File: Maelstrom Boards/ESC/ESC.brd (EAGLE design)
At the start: 101.6 x 101.6 mm, 54 parts, among them P5 MALE1PINHEADER, P6 MALE1PINHEADER, P7 MALE1PINHEADER, P8 MALE1PINHEADER

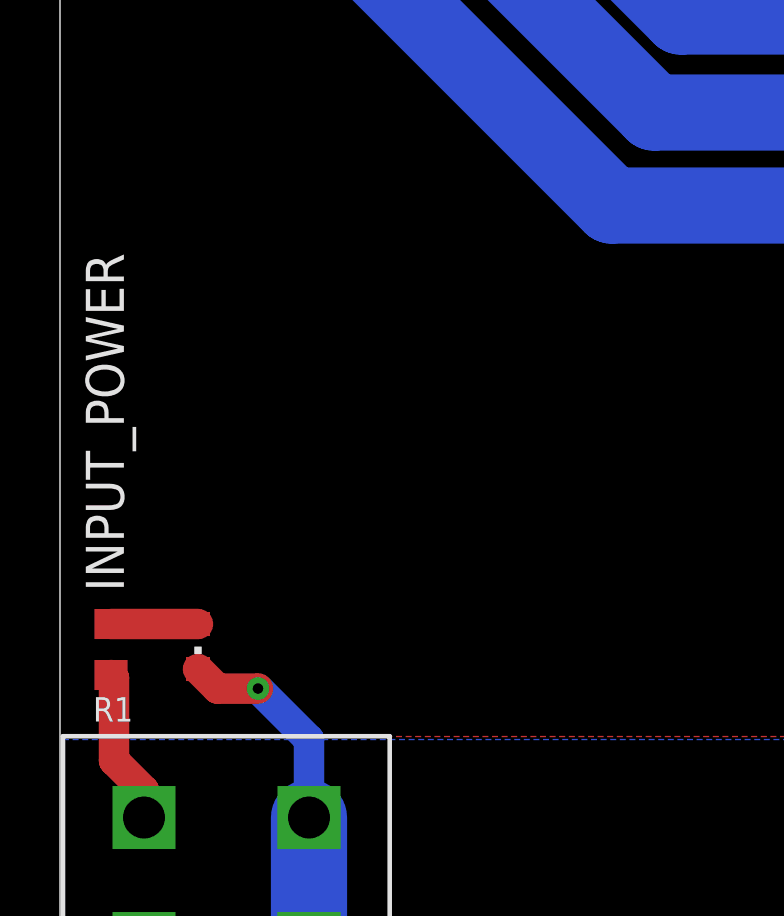
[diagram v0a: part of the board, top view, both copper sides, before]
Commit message: Final changes before order
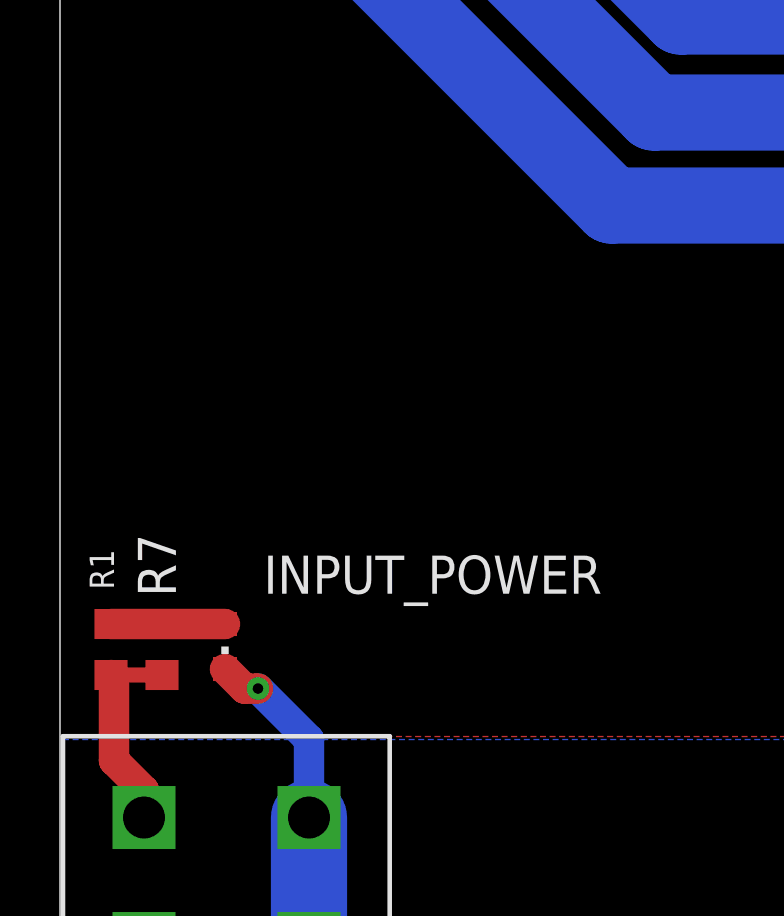
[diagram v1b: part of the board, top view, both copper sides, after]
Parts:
- added R7: 900, resistor:R0603
- R1: value (none) -> 900
- R2: value (none) -> 5
- R3, R4, R5, R6: value (none) -> 100k
- moved INPUT_POWER 0.90 mm to (5.50, 47.0)
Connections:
- net BALANCED+: now also R7.1
- net N$25: now also R7.2
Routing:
- net N$25: track 2.90 -> 5.50 mm
- net BALANCED+: track 5.21 -> 6.91 mm
- net GND: track 149.0 -> 148.1 mm
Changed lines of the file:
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@@
 <layer number="25" name="tNames" color="7" fill="1" visible="yes" active="yes"/>
 <layer number="26" name="bNames" color="7" fill="1" visible="yes" active="yes"/>
-<layer number="27" name="tValues" color="7" fill="1" visible="yes" active="yes"/>
-<layer number="28" name="bValues" color="7" fill="1" visible="yes" active="yes"/>
+<layer number="27" name="tValues" color="7" fill="1" visible="no" active="yes"/>
+<layer number="28" name="bValues" color="7" fill="1" visible="no" active="yes"/>
 <layer number="29" name="tStop" color="7" fill="3" visible="yes" active="yes"/>
 <layer number="30" name="bStop" color="7" fill="6" visible="yes" active="yes"/>
@@
 <text x="98.8" y="24.8" size="0.8128" layer="25">R4</text>
 <text x="30.7" y="8.8" size="0.8128" layer="25">R2</text>
-<text x="1.1" y="44.5" size="0.8128" layer="25">R1</text>
+<text x="1.8" y="48.9" size="0.8128" layer="25" rot="R90">R1</text>
 <text x="83.2" y="11.3" size="1.27" layer="26" rot="MR0">8</text>
 </plain>
@@
 <element name="P8" library="Male_Header_1Pin" package="MALE1PINHEADER" value="MALE1PINHEADER" x="82.55" y="9.652" smashed="yes" rot="R90"/>
 <element name="U$19" library="14_Pin_Connector_Vert" package="14PIN_VERT" value="14PIN_VERT" x="2.8" y="16.1" smashed="yes"/>
-<element name="R1" library="resistor" library_urn="urn:adsk.eagle:library:348" package="R0603" package3d_urn="urn:adsk.eagle:package:26057/1" value="" x="1.7" y="46.9" smashed="yes" rot="R90">
+<element name="R1" library="resistor" library_urn="urn:adsk.eagle:library:348" package="R0603" package3d_urn="urn:adsk.eagle:package:26057/1" value="900" x="1.7" y="46.9" smashed="yes" rot="R90">
 <attribute name="VALUE" x="3.605" y="46.265" size="1.27" layer="27" rot="R90"/>
 </element>
-<element name="R2" library="resistor" library_urn="urn:adsk.eagle:library:348" package="R0603" package3d_urn="urn:adsk.eagle:package:26057/1" value="" x="29.8" y="10.7" smashed="yes">
+<element name="R2" library="resistor" library_urn="urn:adsk.eagle:library:348" package="R0603" package3d_urn="urn:adsk.eagle:package:26057/1" value="5" x="29.8" y="10.7" smashed="yes">
 <attribute name="VALUE" x="29.165" y="8.795" size="1.27" layer="27"/>
 </element>
@@
 <attribute name="VALUE" x="31.53" y="8.795" size="1.27" layer="27"/>
 </element>
-<element name="INPUT_POWER" library="led" library_urn="urn:adsk.eagle:library:259" package="CHIPLED_0603" package3d_urn="urn:adsk.eagle:package:15822/2" value="" x="4.6" y="47" smashed="yes" rot="R180">
-<attribute name="NAME" x="2.13" y="48.835" size="1.27" layer="25" rot="R90"/>
-<attribute name="VALUE" x="2.695" y="48.27" size="1.27" layer="27" rot="R270"/>
+<element name="INPUT_POWER" library="led" library_urn="urn:adsk.eagle:library:259" package="CHIPLED_0603" package3d_urn="urn:adsk.eagle:package:15822/2" value="" x="5.5" y="47" smashed="yes" rot="R180">
+<attribute name="NAME" x="18.065" y="50.03" size="1.27" layer="25" rot="R180"/>
+<attribute name="VALUE" x="3.595" y="48.27" size="1.27" layer="27" rot="R270"/>
 </element>
 <element name="2CONNECT" library="Screw_Terminals" package="1711725" value="1711725" x="19.1" y="19.05" smashed="yes" rot="MR0"/>
@@
 <element name="4C" library="ACS722" package="SOIC-8" value="ACS722" x="48.5" y="18.6" smashed="yes" rot="MR180"/>
 <element name="U$24" library="ADC128D818" package="TSSOP-16" value="ADC128D818" x="94.4" y="21" smashed="yes" rot="R270"/>
-<element name="R3" library="resistor" library_urn="urn:adsk.eagle:library:348" package="R0603" package3d_urn="urn:adsk.eagle:package:26057/1" value="" x="98.7" y="28.8" smashed="yes">
+<element name="R3" library="resistor" library_urn="urn:adsk.eagle:library:348" package="R0603" package3d_urn="urn:adsk.eagle:package:26057/1" value="100k" x="98.7" y="28.8" smashed="yes">
 <attribute name="VALUE" x="98.065" y="26.895" size="1.27" layer="27"/>
 </element>
-<element name="R4" library="resistor" library_urn="urn:adsk.eagle:library:348" package="R0603" package3d_urn="urn:adsk.eagle:package:26057/1" value="" x="98.7" y="26.7" smashed="yes" rot="R180">
+<element name="R4" library="resistor" library_urn="urn:adsk.eagle:library:348" package="R0603" package3d_urn="urn:adsk.eagle:package:26057/1" value="100k" x="98.7" y="26.7" smashed="yes" rot="R180">
 <attribute name="VALUE" x="99.335" y="28.605" size="1.27" layer="27" rot="R180"/>
 </element>
-<element name="R5" library="resistor" library_urn="urn:adsk.eagle:library:348" package="R0603" package3d_urn="urn:adsk.eagle:package:26057/1" value="" x="92.2" y="26.7" smashed="yes">
+<element name="R5" library="resistor" library_urn="urn:adsk.eagle:library:348" package="R0603" package3d_urn="urn:adsk.eagle:package:26057/1" value="100k" x="92.2" y="26.7" smashed="yes">
 <attribute name="VALUE" x="91.565" y="24.795" size="1.27" layer="27"/>
 </element>
-<element name="R6" library="resistor" library_urn="urn:adsk.eagle:library:348" package="R0603" package3d_urn="urn:adsk.eagle:package:26057/1" value="" x="92.2" y="28.8" smashed="yes" rot="R180">
+<element name="R6" library="resistor" library_urn="urn:adsk.eagle:library:348" package="R0603" package3d_urn="urn:adsk.eagle:package:26057/1" value="100k" x="92.2" y="28.8" smashed="yes" rot="R180">
 <attribute name="VALUE" x="92.835" y="30.705" size="1.27" layer="27" rot="R180"/>
 </element>
@@
 <attribute name="SPICEPREFIX" value="C" x="98.7" y="19.5" size="1.778" layer="27" display="off"/>
 </element>
+<element name="R7" library="resistor" library_urn="urn:adsk.eagle:library:348" package="R0603" package3d_urn="urn:adsk.eagle:package:26057/1" value="900" x="3.4" y="46.9" smashed="yes" rot="R90">
+<attribute name="NAME" x="3.865" y="48.665" size="1.27" layer="25" rot="R90"/>
+<attribute name="VALUE" x="5.305" y="46.265" size="1.27" layer="27" rot="R90"/>
+</element>
 </elements>
 <signals>
@@
 <wire x1="6.6" y1="45.6" x2="8.3" y2="43.9" width="1.016" layer="16"/>
 <wire x1="8.3" y1="43.9" x2="8.3" y2="41.3" width="1.016" layer="16"/>
-<wire x1="4.6" y1="46.25" x2="5.25" y2="45.6" width="1.016" layer="1"/>
-<wire x1="5.25" y1="45.6" x2="6.6" y2="45.6" width="1.016" layer="1"/>
+<wire x1="5.5" y1="46.25" x2="6.15" y2="45.6" width="1.016" layer="1"/>
+<wire x1="6.15" y1="45.6" x2="6.6" y2="45.6" width="1.016" layer="1"/>
 <contactref element="8C" pad="GND"/>
 <contactref element="C11" pad="1"/>
@@
 <wire x1="1.8" y1="43.2" x2="1.8" y2="45.95" width="1.016" layer="1"/>
 <wire x1="1.8" y1="45.95" x2="1.7" y2="46.05" width="1.016" layer="1"/>
+<contactref element="R7" pad="1"/>
+<wire x1="1.7" y1="46.05" x2="3.4" y2="46.05" width="0.508" layer="1"/>
 </signal>
 <signal name="PWM_1">
@@
 <contactref element="R1" pad="2"/>
 <contactref element="INPUT_POWER" pad="A"/>
-<wire x1="1.7" y1="47.75" x2="4.6" y2="47.75" width="1.016" layer="1"/>
+<wire x1="1.7" y1="47.75" x2="5.5" y2="47.75" width="1.016" layer="1"/>
+<contactref element="R7" pad="2"/>
+<wire x1="3.4" y1="47.75" x2="1.7" y2="47.75" width="0.1524" layer="1"/>
 </signal>
 <signal name="N$26">
